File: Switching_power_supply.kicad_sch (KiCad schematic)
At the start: 29 parts, among them J8 Conn_01x03_Pin, SW1 SW_DIP_x04, U4 AMS1117, U5 LM2596HVS-ADJRG

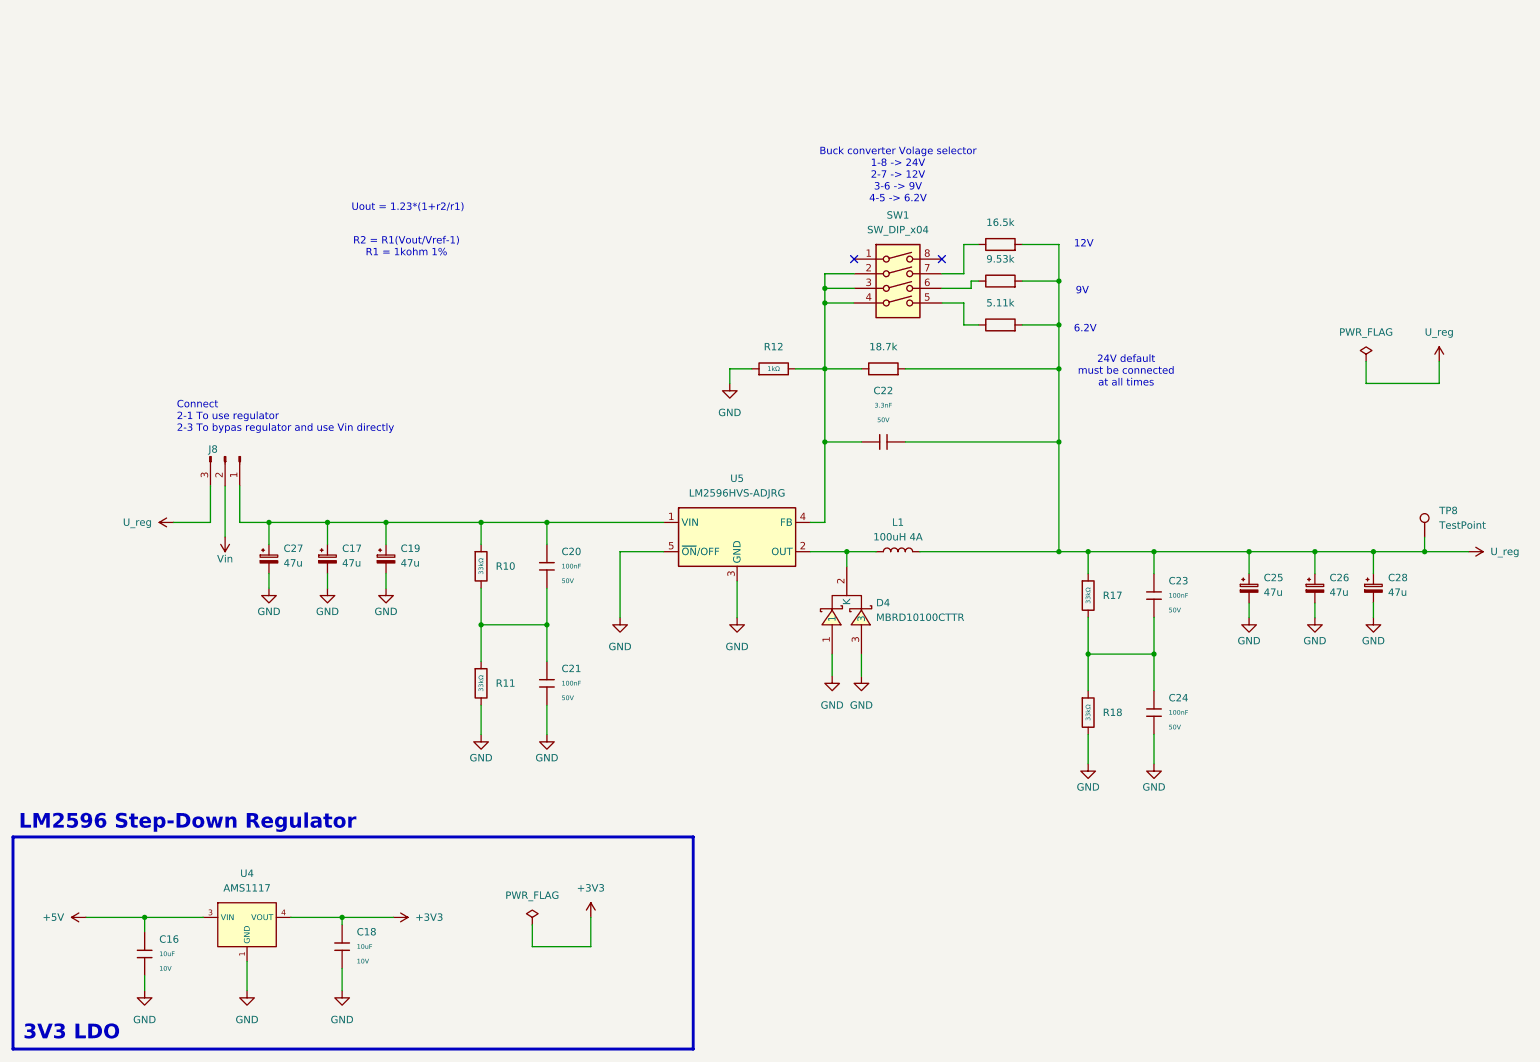
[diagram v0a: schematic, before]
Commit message: minor fixes + production files
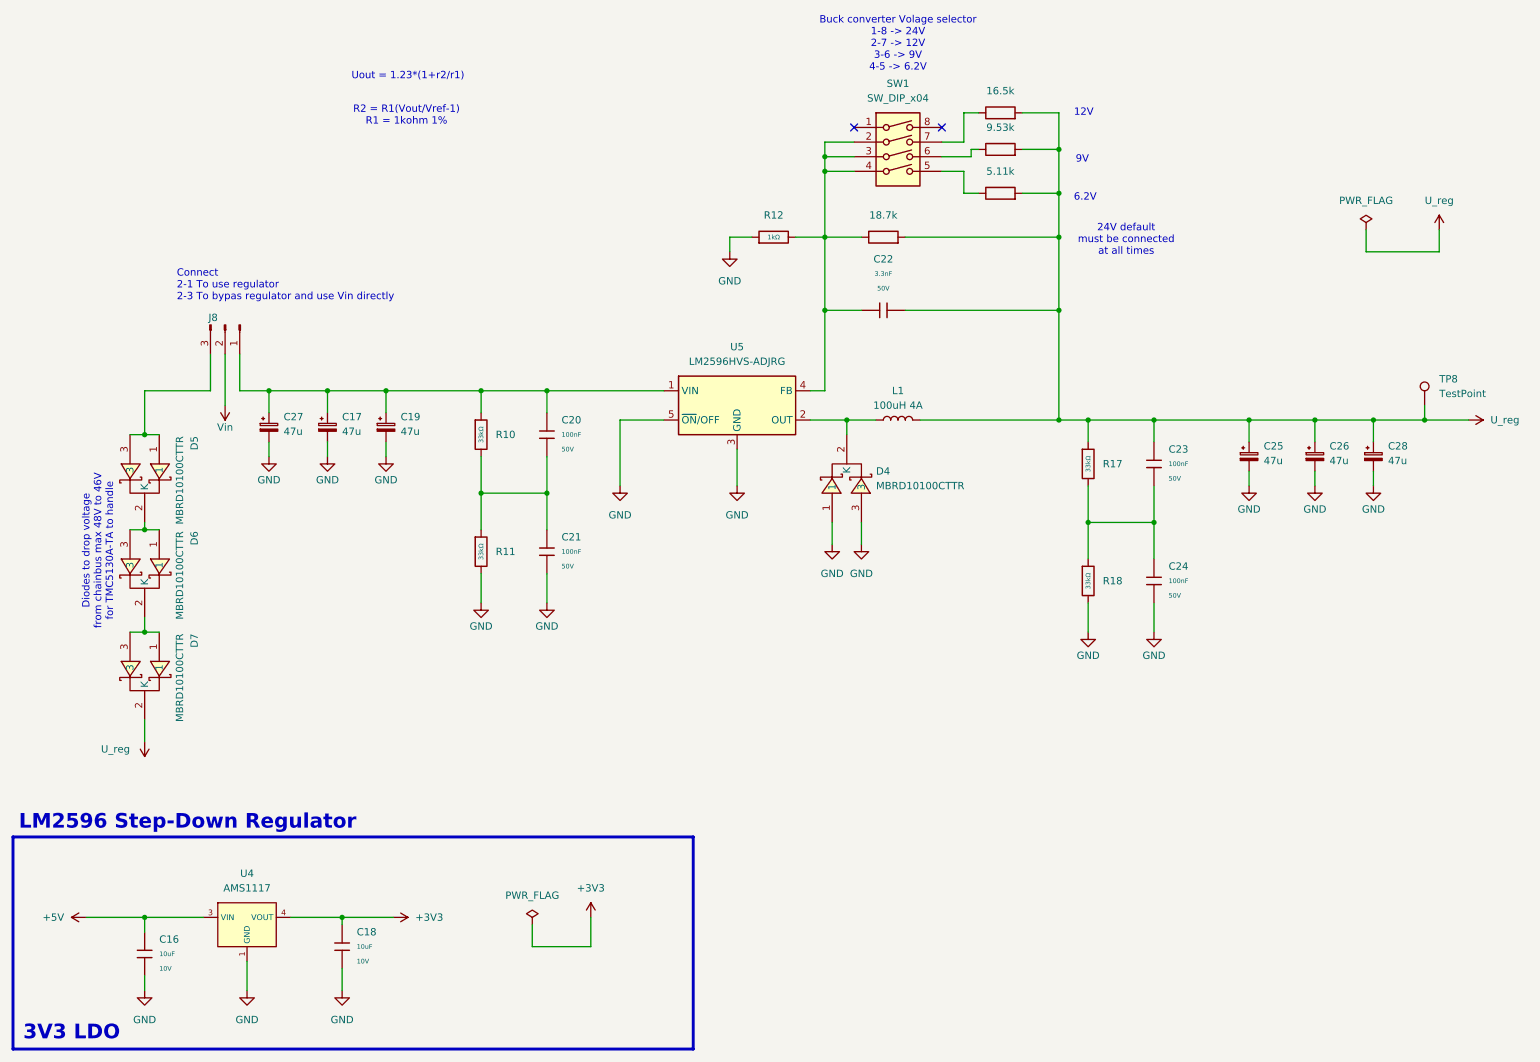
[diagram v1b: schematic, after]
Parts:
- added D5, D6, D7: MBRD10100CTTR, SMC_MBRD10100CTTR:TO-252-3_L6.5-W5.8-P4.58-TL, symbol SMC_MBRD10100CTTR:MBRD10100CTTR
- L1: LCSC C5368704 -> C5368704
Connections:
- net U_reg: now also D7.2 (K); no longer J8.3 (Pin_3)
- new net: D6.2 (K), D7.1, D7.3
- new net: D5.1, D5.3, J8.3 (Pin_3)
- new net: D5.2 (K), D6.1, D6.3
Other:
- note added: "Diodes to drop voltage from chainbus max 48V to 46V for TMC5130A-TA to handle"
- moved on the sheet: C17, C19, C20, C21, C22, C23, C24, C25, C26, C27, C28, D4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
